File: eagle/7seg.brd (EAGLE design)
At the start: 14 parts, among them J1 CONN-8P, J2 CONN-4P-4P

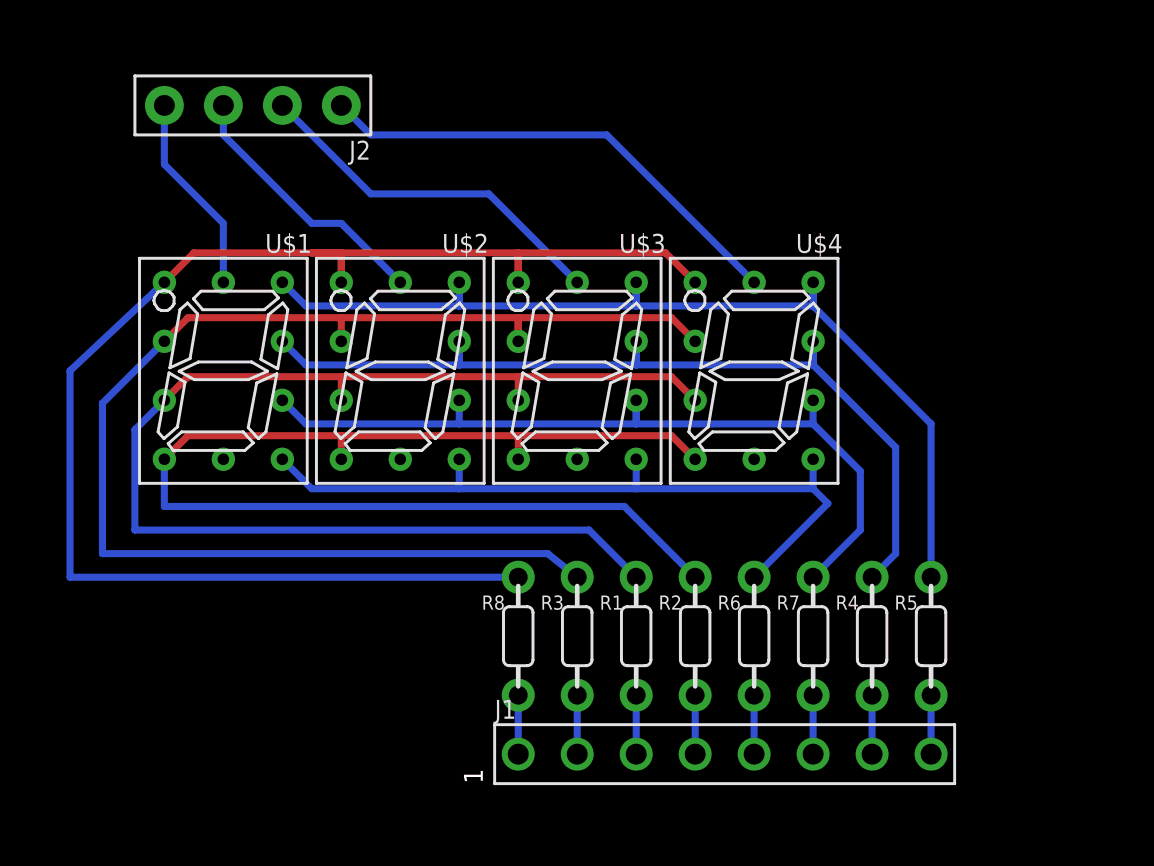
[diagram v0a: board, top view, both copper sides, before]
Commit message: ...
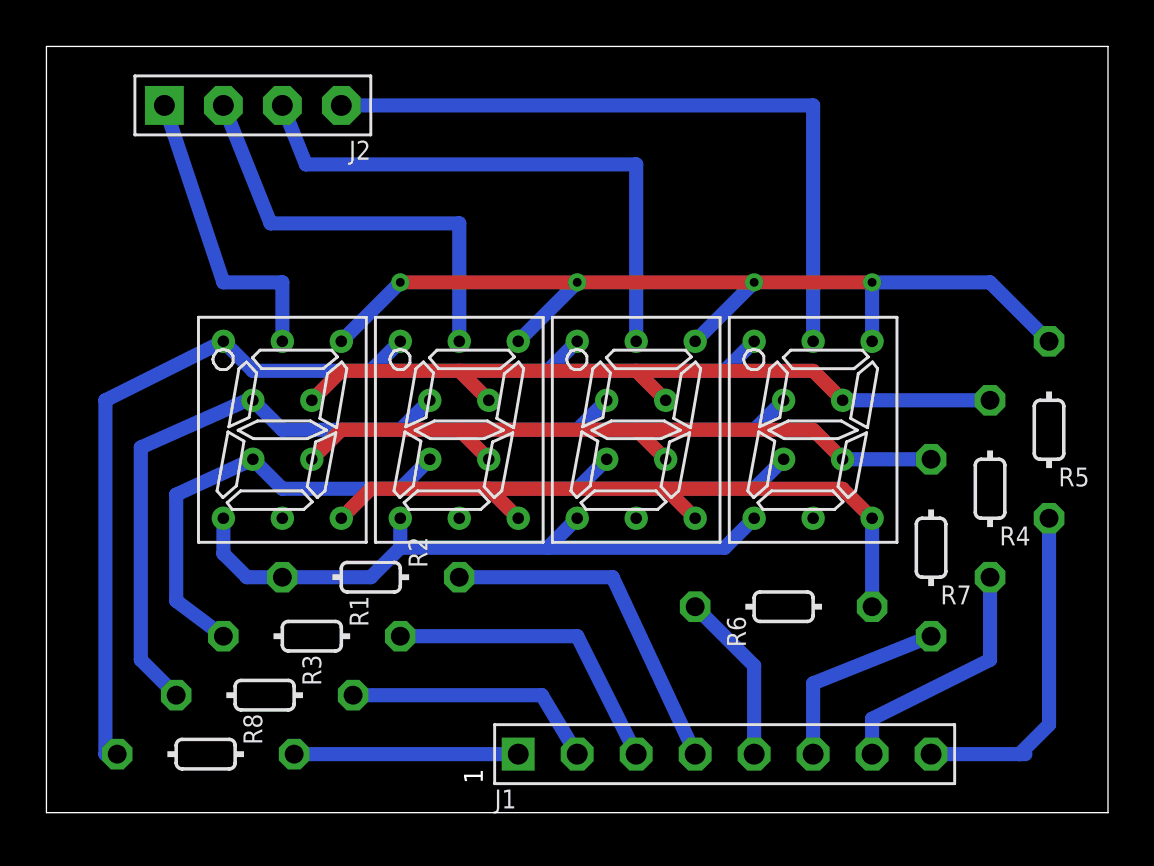
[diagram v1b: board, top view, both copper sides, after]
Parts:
- R1, R2, R3, R4, R5, R6, R7, R8: value 330Ω -> (none); device r:0202/5-V -> r:0202/7-V
- U$1, U$2, U$3, U$4: value TDSO1160-2.54 -> TDSO1160; device lcd:TDSX1150-2.54 -> lcd:TDSX1150
- moved R8 14.4 mm to (6.86, 2.54), turned to 90 degrees
- moved R2 14.2 mm to (14.0, 10.2), turned to 90 degrees
- moved R1 14.0 mm to (11.4, 7.62), turned to 90 degrees
- moved R3 13.7 mm to (9.40, 5.08), turned to 90 degrees
- moved R5 10.2 mm to (43.2, 16.5)
- moved J1 8.89 mm to (29.2, 2.54)
- moved R4 8.13 mm to (40.6, 14.0)
- moved R7 6.35 mm to (38.1, 11.4)
- moved U$4 3.59 mm to (33.0, 16.5)
- moved U$1 3.59 mm to (10.2, 16.5)
- moved U$2 3.59 mm to (17.8, 16.5)
- moved U$3 3.59 mm to (25.4, 16.5)
- moved R6 1.80 mm to (31.8, 8.89), turned to 270 degrees
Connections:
- removed net DP: R8.1, U$1.5, U$2.5, U$3.5, U$4.5
- removed net _A: J1.3, R1.2
- removed net _B: J1.4, R2.2
- removed net _C: J1.2, R3.2
- removed net _D: J1.7, R4.2
- removed net _DP: J1.1, R8.2
- removed net _E: J1.8, R5.2
- removed net _F: J1.5, R6.2
- removed net _G: J1.6, R7.2
- new net N$1: J1.3, R1.1
- new net N$2: J1.4, R2.1
- new net N$3: J1.2, R3.1
- new net N$4: J1.7, R4.1
- new net N$5: J1.8, R5.1
- new net N$6: J1.5, R6.1
- new net N$7: J1.6, R7.1
- new net N$8: J1.1, R8.1
- new net P: R8.2, U$1.5, U$2.5, U$3.5, U$4.5
- net A: now also R1.2; no longer R1.1
- net B: now also R2.2; no longer R2.1
- net C: now also R3.2; no longer R3.1
- net D: now also R4.2; no longer R4.1
- net E: now also R5.2; no longer R5.1
- net F: now also R6.2; no longer R6.1
- net G: now also R7.2; no longer R7.1
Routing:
- net DP: track 65.3 -> 0.00 mm
- net P: track 0.00 -> 48.9 mm
- net B: track 51.9 -> 28.9 mm
- net A: track 54.3 -> 38.3 mm
- net N$2: track 0.00 -> 15.0 mm
- net N$5: track 0.00 -> 14.8 mm
- net C: track 57.8 -> 44.1 mm
- net N$1: track 0.00 -> 13.3 mm
- net N$3: track 0.00 -> 11.1 mm
- net N$4: track 0.00 -> 10.8 mm
- net N$8: track 0.00 -> 9.65 mm
- net C4: track 20.9 -> 30.5 mm
- net C3: track 15.9 -> 24.6 mm
- net N$7: track 0.00 -> 8.52 mm
- net N$6: track 0.00 -> 7.40 mm
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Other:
- board outline added: 45.7 x 33 mm
